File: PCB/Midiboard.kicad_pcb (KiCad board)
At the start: 2 copper layers, 104 x 87 mm, 11 parts, among them J1 Capacitive_keys, SW1 SW_Push, SW2 SW_Push, SW3 SW_Push, SW4 RotaryEncoder_Switch_MP, U1 Waveshare ESP32-S3-ZERO

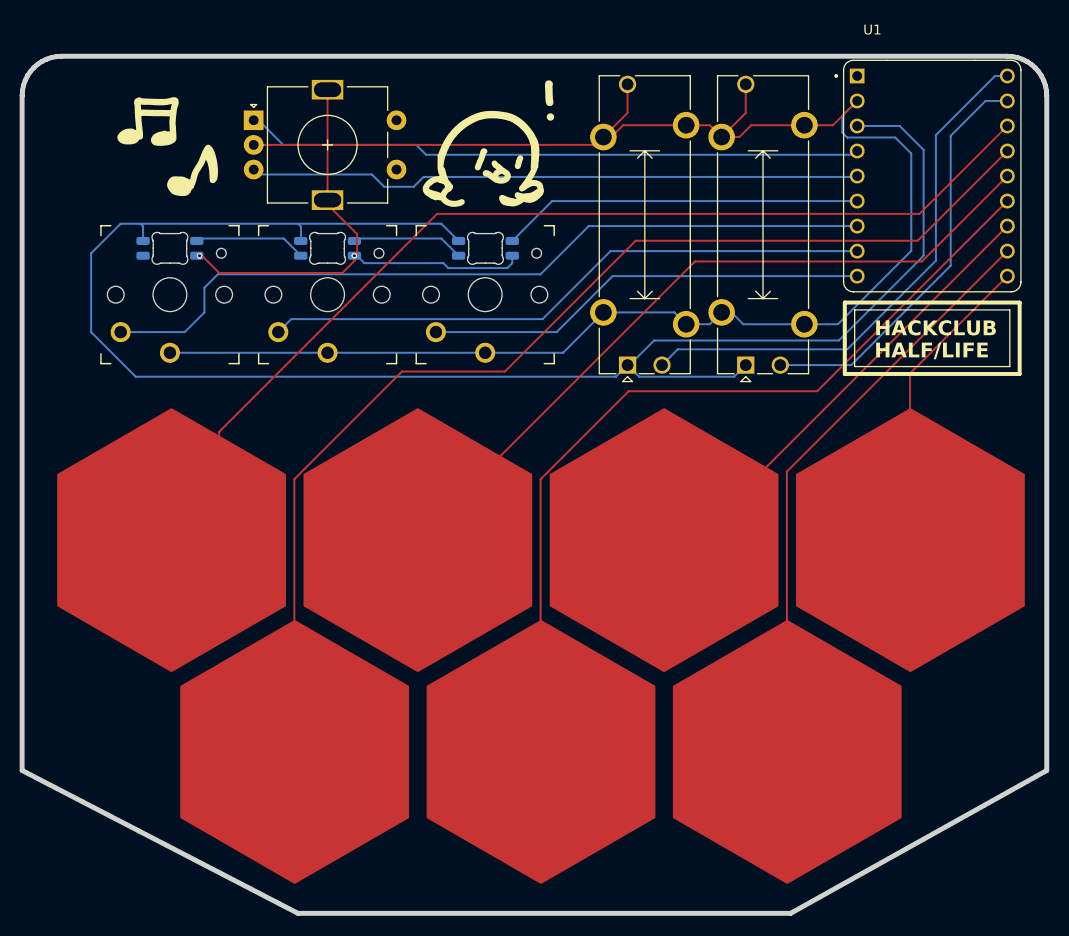
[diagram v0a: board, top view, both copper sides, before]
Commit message: Add files via upload
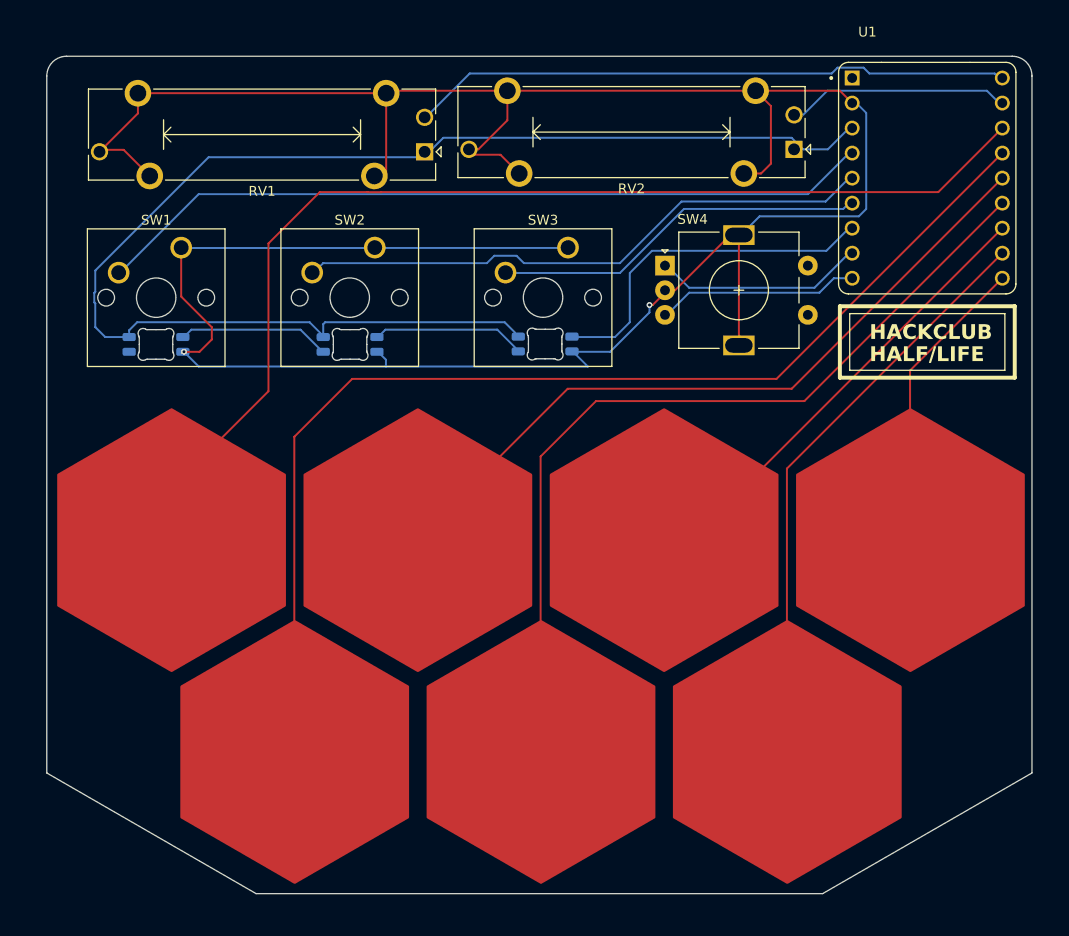
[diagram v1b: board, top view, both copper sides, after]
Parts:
- RV1, RV2: footprint Potentiometer_THT:Potentiometer_Bourns_PTA1543_Single_Slide -> Potentiometer_THT:Potentiometer_Bourns_PTA2043_Single_Slide
- SW1, SW2, SW3: footprint Hackclub Footprints:Kailh Choc Low-Profile Switches -> Button_Switch_Keyboard:SW_Cherry_MX_1.00u_PCB
- moved SW4 44.3 mm to (155.2, 52.2)
- moved RV1 29.9 mm to (130.8, 40.7), turned to 180 degrees
- moved RV2 22.4 mm to (168.3, 40.5), turned to 180 degrees
- moved D1 11.4 mm to (143.1, 60.2)
- moved D2 10.0 mm to (123.3, 60.2)
- moved D3 9.85 mm to (103.6, 60.2)
- moved SW3 9.67 mm to (145.4, 50.4)
- moved SW2 6.77 mm to (125.8, 50.4)
- moved SW1 4.91 mm to (106.1, 50.4)
- moved U1 0.55 mm to (181.9, 43.4)
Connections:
- U1 pad 1: /ENC1_A -> /SWITCH1
- U1 pad 2: /ENC1_B -> /SWITCH2
- U1 pad 3: /LED -> /SWITCH3
- U1 pad 4: /SWITCH1 -> /LED
- U1 pad 5: /SWITCH2 -> /ENC1_A
- U1 pad 6: /SWITCH3 -> /ENC1_B
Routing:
- net GND: track 233.1 -> 281.7 mm
- net /ENC1_B: track 63.1 -> 20.0 mm
- net /ENC1_A: track 63.6 -> 20.9 mm
- net +3V3: track 173.3 -> 137.8 mm
- net /SLIDE2: track 41.9 -> 21.4 mm
- net /SWITCH3: track 45.1 -> 37.7 mm
- net /SLIDE1: track 54.7 -> 60.9 mm
- net Net-(D1-DOUT): track 11.4 -> 15.6 mm
- net Net-(D2-DOUT): track 11.3 -> 15.5 mm
- net /SWITCH2: track 62.2 -> 59.0 mm
- net /TOUCH1: track 116.8 -> 114.0 mm
- net /TOUCH2: track 113.7 -> 116.3 mm
- net /SWITCH1: track 80.7 -> 79.1 mm
- net /TOUCH4: track 86.6 -> 88.0 mm
- net /LED: track 36.7 -> 35.5 mm
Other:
- board size 104 x 87 mm -> 100 x 85 mm
